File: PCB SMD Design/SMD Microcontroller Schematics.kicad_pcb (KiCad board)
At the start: 2 copper layers, 79.9 x 169.5 mm, 49 parts, among them J1 Power (9v), J10 Micro_SD_Card, J11 Throttle HallEffect, J12 Screen Connector, J13 Button 1, J14 Button 2, J15 Button 3, J16 Button 4, J17 Power OUT (9v), J18 Data (RX TX), J19 Power (9v), J2 Data (RX TX), J20 HC12, J21 Rotary SW, J3 Current Sensor, J4 Bat 1V, J5 Bat 1+2 V, J6 RPM Sensor, J7 Motor Temp, J8 Motor Controller Temp, J9 Motor Controller, U1 ESP32-DEVKIT-V1, U2 MCP6002-xP, U3 ADS1115IDGS, U4 ADS1115IDGS, U5 PC817, U6 ESP32-DEVKIT-V1

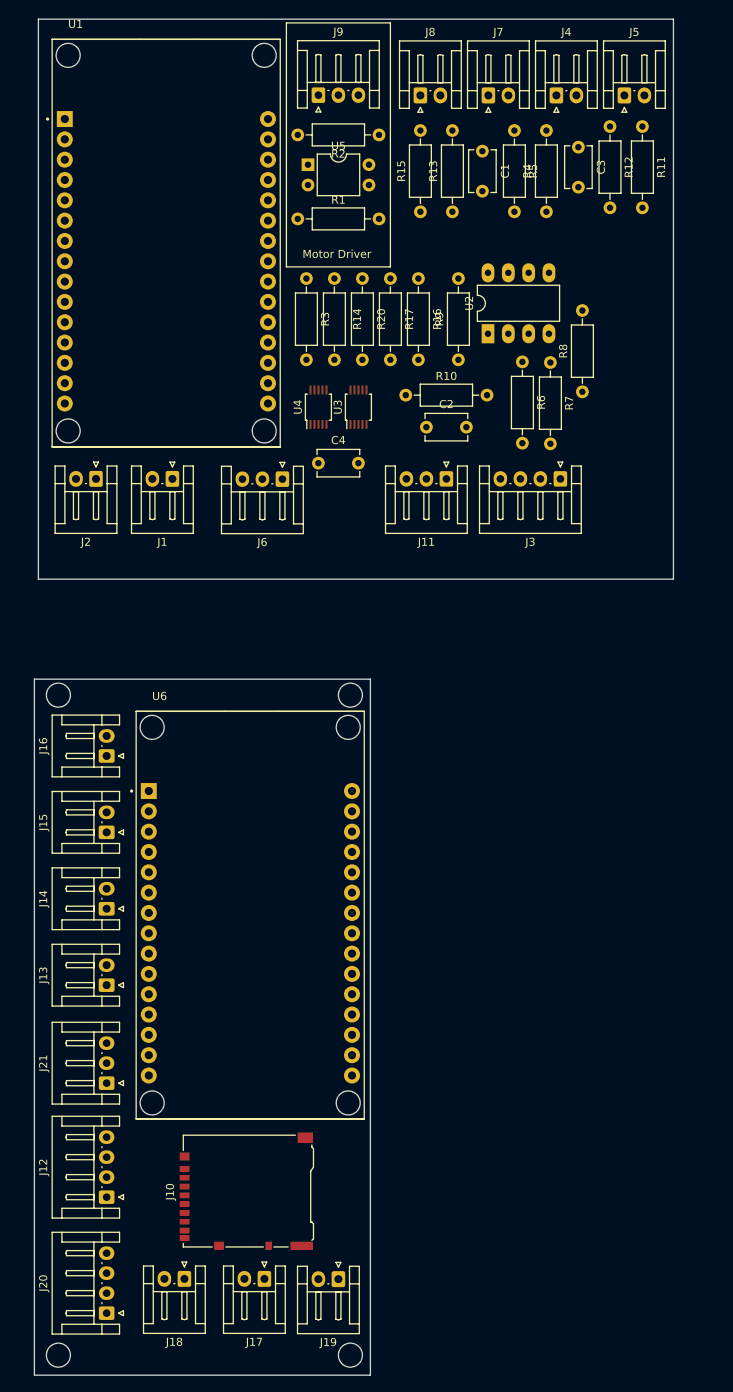
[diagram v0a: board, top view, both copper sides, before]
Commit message: PCB changes
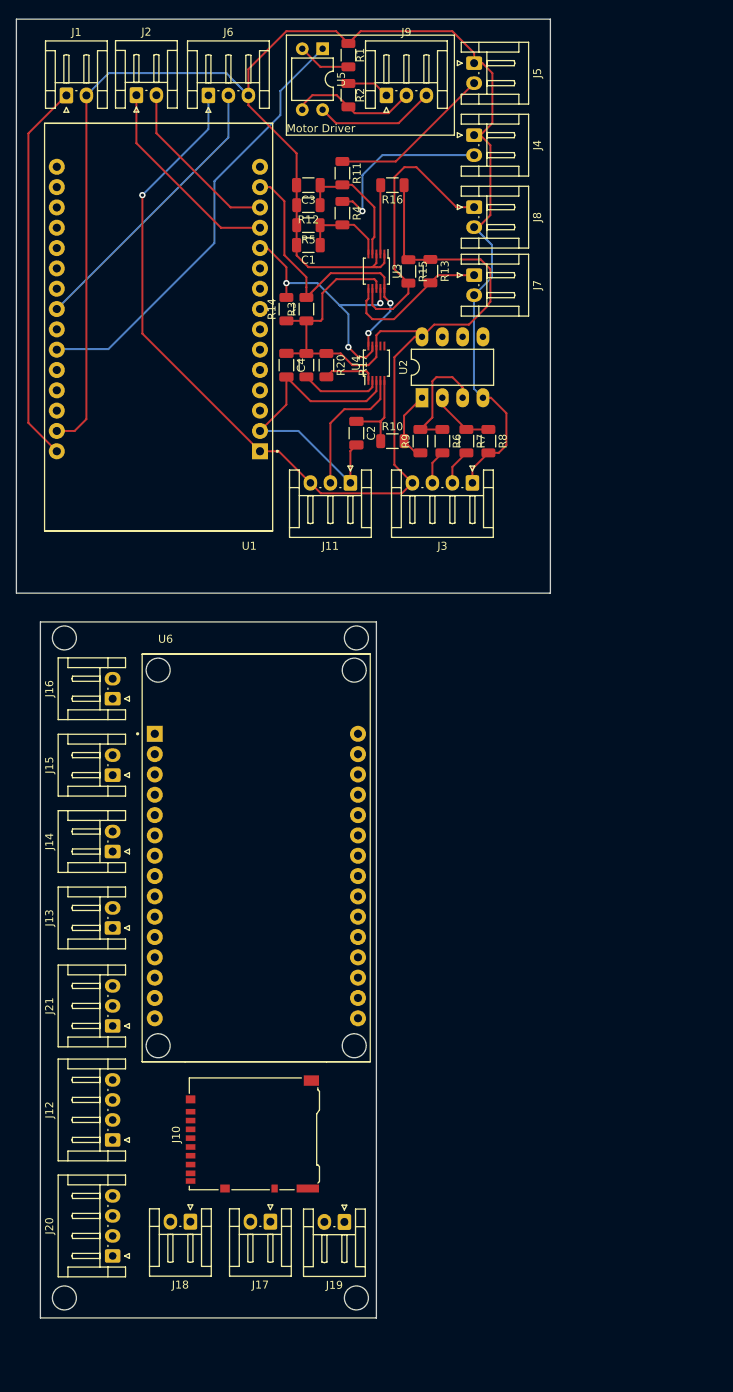
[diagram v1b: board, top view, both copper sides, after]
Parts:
- C1, C2, C3, C4: footprint Capacitor_THT:C_Disc_D5.1mm_W3.2mm_P5.00mm -> Capacitor_SMD:C_1206_3216Metric
- R1, R10, R11, R12, R13, R14, R15, R16, R17, R2, R20, R3, R4, R5, R6, R7, R8, R9: footprint Resistor_THT:R_Axial_DIN0207_L6.3mm_D2.5mm_P10.16mm_Horizontal -> Resistor_SMD:R_1206_3216Metric
- moved J1 49.7 mm to (27.0, 31.0), turned to 0 degrees
- moved J6 48.9 mm to (44.8, 31.0), turned to 0 degrees
- moved J2 48.2 mm to (35.8, 31.0), turned to 0 degrees
- moved R12 39.0 mm to (57.2, 44.8), turned to 180 degrees
- moved R11 38.0 mm to (61.5, 40.8)
- moved C3 34.1 mm to (57.2, 42.2), turned to 180 degrees
- moved R5 28.3 mm to (57.2, 47.2), turned to 180 degrees
- moved R4 25.5 mm to (61.5, 45.8), turned to -90 degrees
- moved C1 24.7 mm to (57.2, 49.8), turned to 180 degrees
- moved J7 22.5 mm to (78.0, 53.5), turned to -90 degrees
- moved R1 21.4 mm to (62.2, 26.0), turned to -90 degrees
- moved J5 19.2 mm to (78.0, 27.0), turned to -90 degrees
- moved U3 17.1 mm to (65.8, 53.0), turned to -90 degrees
- moved J8 15.5 mm to (78.0, 45.0), turned to -90 degrees
- moved R17 15.1 mm to (57.0, 64.8)
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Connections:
- net Net-(J9-Pin_2) renamed /Data
- J3 pad 4: +5V -> 3.3V
- U2 pad 8: +5V -> 3.3V
- U4 pad 4: Current -> Net-(J11-Pin_2)
- U4 pad 5: Net-(J11-Pin_2) -> Current
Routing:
- net GND: track 0.00 -> 247.1 mm
- net 3.3V: track 0.00 -> 173.6 mm, vias 0 -> 1
- net GPIO 27 - PWM: track 0.00 -> 55.1 mm
- net 9V: track 0.00 -> 47.9 mm
- net SCL: track 0.00 -> 38.3 mm, vias 0 -> 2
- net Net-(J6-Pin_2): track 0.00 -> 35.6 mm
- net Motor Controller Temp: track 0.00 -> 35.4 mm
- net SDA: track 0.00 -> 33.1 mm, vias 0 -> 3
- net Net-(J2-Pin_1): track 0.00 -> 25.8 mm
- net Net-(J4-Pin_2): track 0.00 -> 22.5 mm, vias 0 -> 1
- net Net-(J2-Pin_2): track 0.00 -> 21.5 mm
- net Net-(J5-Pin_2): track 0.00 -> 20.5 mm
- net Motor Temp: track 0.00 -> 19.3 mm
- net Net-(J11-Pin_2): track 0.00 -> 17.3 mm
- net Reduced TotalV: track 0.00 -> 16.5 mm
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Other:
- board size 79.9 x 169.5 mm -> 66.8 x 162.3 mm

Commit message: Many Changes
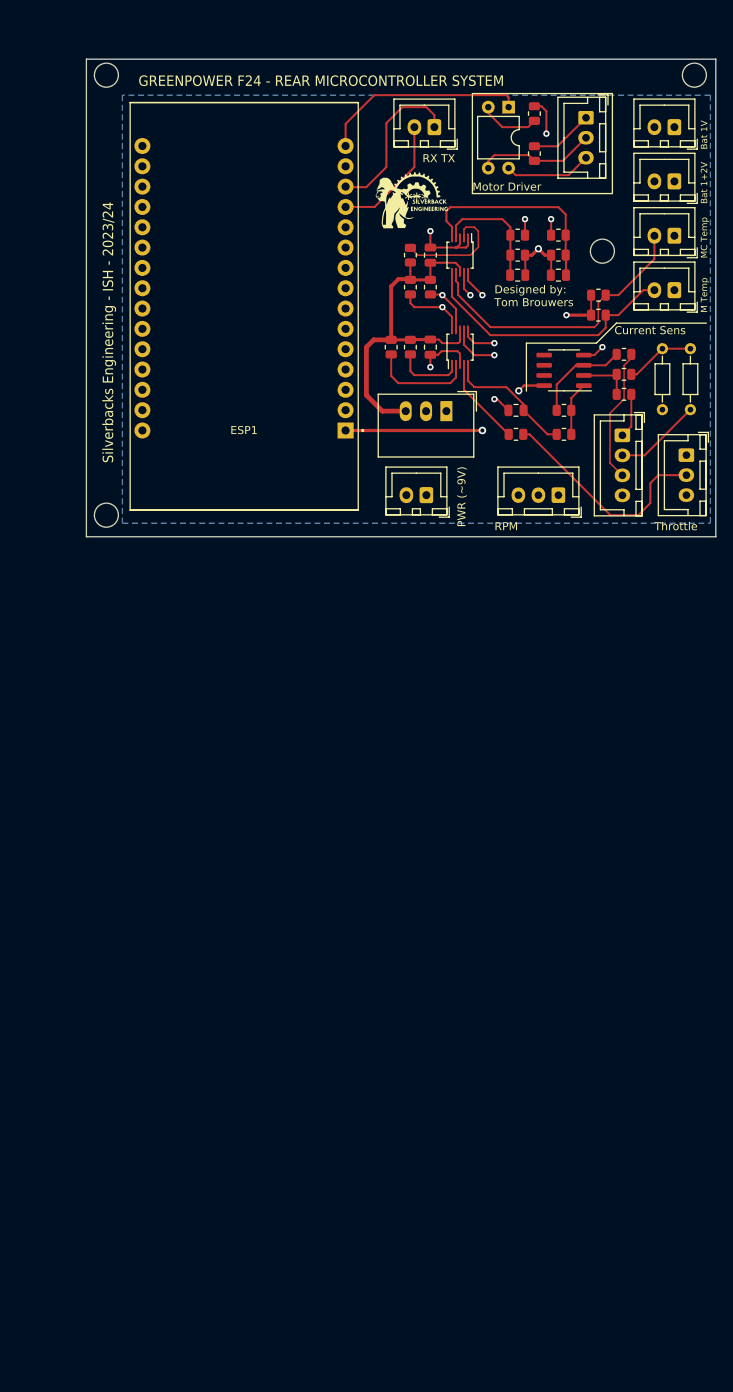
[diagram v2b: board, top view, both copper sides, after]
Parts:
- removed the J10 at (50.2, 160.8)
- removed J12: Screen Connector, Connector_JST:JST_EH_S4B-EH_1x04_P2.50mm_Horizontal
- removed J13: Button 1, Connector_JST:JST_EH_S2B-EH_1x02_P2.50mm_Horizontal
- removed J14: Button 2, Connector_JST:JST_EH_S2B-EH_1x02_P2.50mm_Horizontal
- removed J15: Button 3, Connector_JST:JST_EH_S2B-EH_1x02_P2.50mm_Horizontal
- removed J16: Button 4, Connector_JST:JST_EH_S2B-EH_1x02_P2.50mm_Horizontal
- removed J17: Power OUT (9v), Connector_JST:JST_EH_S2B-EH_1x02_P2.50mm_Horizontal
- removed J18: Data (RX TX), Connector_JST:JST_EH_S2B-EH_1x02_P2.50mm_Horizontal
- removed J19: Power (9v), Connector_JST:JST_EH_S2B-EH_1x02_P2.50mm_Horizontal
- removed J20: HC12, Connector_JST:JST_EH_S4B-EH_1x04_P2.50mm_Horizontal
- removed J21: Rotary SW, Connector_JST:JST_EH_S3B-EH_1x03_P2.50mm_Horizontal
- removed the J8 at (78.0, 45.0)
- removed U6: ESP32-DEVKIT-V1, ESP32-DEVKIT-V1:MODULE_ESP32_DEVKIT_V1
- added C5: 100nF, Capacitor_SMD:C_0805_2012Metric, F.Cu at (72.5, 62.5)
- added G***: LOGO, SC0915:SBX_Logo, F.Cu at (70.0, 44.0)
- added J6: Motor Temp, Connector_JST:JST_XH_B2B-XH-A_1x02_P2.50mm_Vertical, F.Cu at (103.0, 55.4)
- added R14: 1k, Resistor_SMD:R_0805_2012Metric, F.Cu at (83.2, 73.4)
- added R15: 10k, Resistor_SMD:R_0805_2012Metric, F.Cu at (67.6, 62.5)
- added R21: ?, Resistor_THT:R_Axial_DIN0204_L3.6mm_D1.6mm_P7.62mm_Horizontal, F.Cu at (101.5, 70.3)
- added U1: TSR_1-2450, Converter_DCDC:Converter_DCDC_TRACO_TSR-1_THT, F.Cu at (74.5, 70.5)
- C1, C4: footprint Capacitor_SMD:C_1206_3216Metric -> Capacitor_SMD:C_0805_2012Metric
- C2: renamed from C3; footprint Capacitor_SMD:C_1206_3216Metric -> Capacitor_SMD:C_0805_2012Metric
- C3: renamed from C2; footprint Capacitor_SMD:C_1206_3216Metric -> Capacitor_SMD:C_0805_2012Metric
- J1, J2, J4, J5: footprint Connector_JST:JST_EH_S2B-EH_1x02_P2.50mm_Horizontal -> Connector_JST:JST_XH_B2B-XH-A_1x02_P2.50mm_Vertical
- J10: renamed from J11; footprint Connector_JST:JST_EH_S3B-EH_1x03_P2.50mm_Horizontal -> Connector_JST:JST_XH_B3B-XH-A_1x03_P2.50mm_Vertical
- J3: renamed from J6; footprint Connector_JST:JST_EH_S3B-EH_1x03_P2.50mm_Horizontal -> Connector_JST:JST_XH_B3B-XH-A_1x03_P2.50mm_Vertical
- J7: value Motor Temp -> Motor Controller Temp; footprint Connector_JST:JST_EH_S2B-EH_1x02_P2.50mm_Horizontal -> Connector_JST:JST_XH_B2B-XH-A_1x02_P2.50mm_Vertical
- J8: renamed from J3; footprint Connector_JST:JST_EH_S4B-EH_1x04_P2.50mm_Horizontal -> Connector_JST:JST_XH_B4B-XH-A_1x04_P2.50mm_Vertical
- J9: footprint Connector_JST:JST_EH_S3B-EH_1x03_P2.50mm_Horizontal -> Connector_JST:JST_XH_B3B-XH-A_1x03_P2.50mm_Vertical
- R1: renamed from R4; footprint Resistor_SMD:R_1206_3216Metric -> Resistor_SMD:R_0805_2012Metric
- R10: renamed from R9; footprint Resistor_SMD:R_1206_3216Metric -> Resistor_SMD:R_0805_2012Metric
- R11: renamed from R10; footprint Resistor_SMD:R_1206_3216Metric -> Resistor_SMD:R_0805_2012Metric
- R12: renamed from R2; footprint Resistor_SMD:R_1206_3216Metric -> Resistor_SMD:R_0805_2012Metric
- R13: renamed from R1; footprint Resistor_SMD:R_1206_3216Metric -> Resistor_SMD:R_0805_2012Metric
- R16, R17: footprint Resistor_SMD:R_1206_3216Metric -> Resistor_SMD:R_0805_2012Metric
- R18: renamed from R3; footprint Resistor_SMD:R_1206_3216Metric -> Resistor_SMD:R_0805_2012Metric
- R19: renamed from R14; footprint Resistor_SMD:R_1206_3216Metric -> Resistor_SMD:R_0805_2012Metric
- R2: renamed from R5; footprint Resistor_SMD:R_1206_3216Metric -> Resistor_SMD:R_0805_2012Metric
- R20: value 10k -> ?; footprint Resistor_SMD:R_1206_3216Metric -> Resistor_THT:R_Axial_DIN0204_L3.6mm_D1.6mm_P7.62mm_Horizontal
- R3: renamed from R11; footprint Resistor_SMD:R_1206_3216Metric -> Resistor_SMD:R_0805_2012Metric
- R4: renamed from R12; footprint Resistor_SMD:R_1206_3216Metric -> Resistor_SMD:R_0805_2012Metric
- R5: renamed from R13; footprint Resistor_SMD:R_1206_3216Metric -> Resistor_SMD:R_0805_2012Metric
- R6: renamed from R15; footprint Resistor_SMD:R_1206_3216Metric -> Resistor_SMD:R_0805_2012Metric
- R7: renamed from R6; footprint Resistor_SMD:R_1206_3216Metric -> Resistor_SMD:R_0805_2012Metric
- R8: renamed from R7; footprint Resistor_SMD:R_1206_3216Metric -> Resistor_SMD:R_0805_2012Metric
- R9: renamed from R8; footprint Resistor_SMD:R_1206_3216Metric -> Resistor_SMD:R_0805_2012Metric
- U2: value MCP6002-xP -> MCP6002DRG; footprint Package_DIP:DIP-8_W7.62mm_LongPads -> Package_SO:SOIC-8_3.9x4.9mm_P1.27mm
- moved J1 67.2 mm to (72.0, 81.0), turned to 180 degrees
- moved J3 66.4 mm to (88.5, 81.0), turned to 180 degrees
- moved R20 45.8 mm to (105.0, 70.3), turned to 90 degrees
- moved J10 42.1 mm to (104.5, 76.0), turned to -90 degrees
- moved J2 37.5 mm to (73.0, 35.0), turned to 180 degrees
- moved C2 33.2 mm to (88.5, 53.5)
- moved R4 31.9 mm to (88.5, 51.0)
- moved J5 29.1 mm to (103.0, 41.8), turned to 180 degrees
- moved R3 28.1 mm to (88.5, 48.5), turned to 0 degrees
- moved C1 26.4 mm to (83.4, 53.5), turned to 0 degrees
- moved R2 26.4 mm to (83.4, 51.0), turned to 0 degrees
- moved J7 25.5 mm to (103.0, 48.6), turned to 180 degrees
- moved R7 25.2 mm to (96.7, 63.4), turned to 0 degrees
- moved J9 25.1 mm to (92.0, 33.8), turned to -90 degrees
- moved J4 25.1 mm to (103.0, 35.0), turned to 180 degrees
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- renumbered U1 to ESP1, U5 to U3, U3 to U4, U4 to U5
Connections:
- net Net-(J9-Pin_1) renamed /MotorGND
- net Net-(J9-Pin_3) renamed /Motor5V
- C4 pad 1: 3.3V -> 5V
- ESP1 pad 10: unconnected-(U1-D19-Pad10) -> GP19
- ESP1 pad 12: Net-(J2-Pin_1) -> Net-(ESP1-RX0)
- ESP1 pad 13: Net-(J2-Pin_2) -> Net-(ESP1-TX0)
- ESP1 pad 15: unconnected-(U1-D23-Pad15) -> GPIO 27 - PWM
- ESP1 pad 19: unconnected-(U1-D34-Pad19) -> /D34
- ESP1 pad 20: unconnected-(U1-D35-Pad20) -> /D35
- ESP1 pad 21: unconnected-(U1-D32-Pad21) -> /D32
- ESP1 pad 22: unconnected-(U1-D33-Pad22) -> /D33
- ESP1 pad 23: Net-(J6-Pin_2) -> /D25
- ESP1 pad 24: unconnected-(U1-D26-Pad24) -> /D26
- ESP1 pad 25: GPIO 27 - PWM -> /D27
- ESP1 pad 26: unconnected-(U1-D14-Pad26) -> Net-(ESP1-D14)
- ESP1 pad 27: unconnected-(U1-D12-Pad27) -> Net-(ESP1-D12)
- ESP1 pad 28: unconnected-(U1-D13-Pad28) -> Net-(ESP1-D13)
- ESP1 pad 3: unconnected-(U1-D15-Pad3) -> Net-(ESP1-D15)
- ESP1 pad 4: unconnected-(U1-D2-Pad4) -> Net-(ESP1-D2)
- ESP1 pad 5: unconnected-(U1-D4-Pad5) -> Net-(ESP1-D4)
- ESP1 pad 8: unconnected-(U1-D5-Pad8) -> Net-(ESP1-D5)
- ESP1 pad 9: unconnected-(U1-D18-Pad9) -> Net-(ESP1-D18)
- J1 pad 1: 9V -> GND
- J1 pad 2: GND -> 9V
- J10 pad 2: Net-(J11-Pin_2) -> Net-(J10-Pin_2)
- J10 pad 3: 3.3V -> 5V
- J2 pad 1: Net-(J2-Pin_1) -> Net-(ESP1-TX0)
- J2 pad 2: Net-(J2-Pin_2) -> Net-(ESP1-RX0)
- J3 pad 1: 3.3V -> GND
- J3 pad 2: Net-(J6-Pin_2) -> GP19
- J3 pad 3: GND -> 3.3V
- J7 pad 1: Motor Temp -> GND
- J7 pad 2: GND -> Motor Controller Temp
- J8 pad 2: Net-(J3-Pin_2) -> Net-(J8-Pin_2)
- J8 pad 4: 3.3V -> 5V
- R16 pad 1: 3.3V -> 5V
- R17 pad 1: 3.3V -> 5V
- R17 pad 2: Net-(U4-ALERT/RDY) (its old number) -> Net-(U5-ADDR)
- R18 pad 1: 3.3V -> 5V
- R19 pad 1: 3.3V -> 5V
- R20 pad 1: 3.3V -> Net-(J8-Pin_2)
- R20 pad 2: Net-(U4-ADDR) -> Net-(R20-Pad2)
- R8 pad 2: Net-(J3-Pin_2) -> Net-(R20-Pad2)
- U2 pad 8: 3.3V -> 5V
- U4 pad 4: Reduced TotalV -> Reduced Bat1V
- U4 pad 5: Reduced Bat1V -> Reduced TotalV
- U4 pad 8: 3.3V -> 5V
- U5 pad 1: Net-(U4-ADDR) -> Net-(U5-ADDR)
- U5 pad 2: Net-(U4-ALERT/RDY) (its old number) -> Net-(U5-ALERT/RDY)
- U5 pad 4: Net-(J11-Pin_2) -> Net-(U5-AIN0)
- U5 pad 8: 3.3V -> 5V
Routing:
- net GND: track 247.1 -> 41.3 mm, vias 0 -> 8
- net 3.3V: track 173.6 -> 51.4 mm, vias 1 -> 2
- net 5V: track 0.00 -> 95.0 mm, vias 0 -> 1
- net GP19: track 0.00 -> 50.1 mm
- net Net-(J6-Pin_2): track 35.6 -> 0.00 mm
- net GPIO 27 - PWM: track 55.1 -> 26.0 mm
- net Net-(J10-Pin_2): track 0.00 -> 28.1 mm
- net Net-(J2-Pin_1): track 25.8 -> 0.00 mm
- net Net-(J2-Pin_2): track 21.5 -> 0.00 mm
- net Net-(ESP1-TX0): track 0.00 -> 20.4 mm
- net Net-(J11-Pin_2): track 17.3 -> 0.00 mm
- net Net-(ESP1-RX0): track 0.00 -> 15.7 mm
- net Motor Temp: track 19.3 -> 33.7 mm
- net Net-(U5-ALERT/RDY): track 0.00 -> 13.2 mm
- net Net-(J8-Pin_3): track 4.27 -> 16.9 mm
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- added copper zone on B.Cu, net GND
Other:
- board size 66.8 x 162.3 mm -> 78.7 x 59.7 mm
- copper layers 2 -> 4
- board text added: "Bat 1+2V"
- board text added: "Bat 1V"
- board text added: "Current Sens"
- board text added: "Designed by: Tom Brouwers"
- board text added: "GREENPOWER F24 - REAR MICROCONTROLLER SYSTEM"
- board text added: "M Temp"
- board text added: "MC Temp"
- board text added: "PWR (~9V)"
- board text added: "RPM"
- board text added: "RX TX"
- board text added: "Silverbacks Engineering - ISH - 2023/24"
- board text added: "Throttle"
